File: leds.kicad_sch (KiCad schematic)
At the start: 12 parts

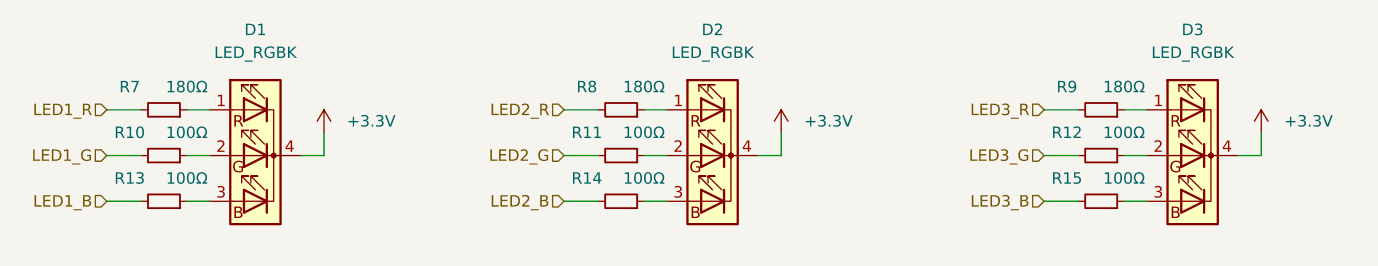
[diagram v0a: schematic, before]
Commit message: Improve DCDC converter diagram
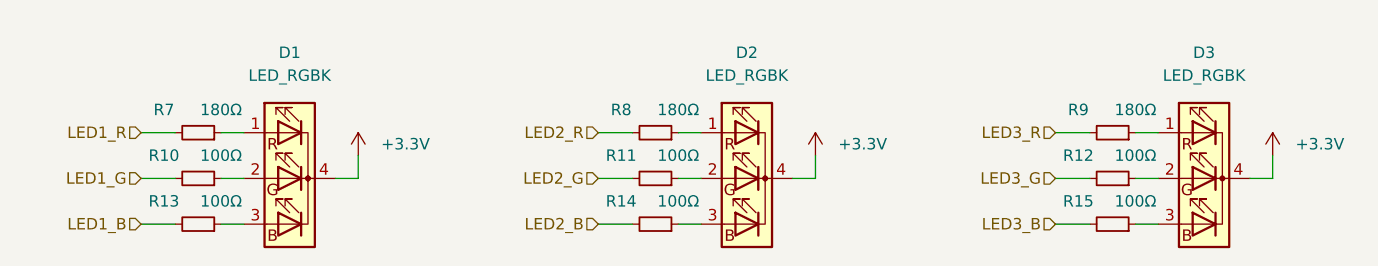
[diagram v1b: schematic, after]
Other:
- company: (none) -> Authors: A. Kotkov, I. Kajdan
- title: (none) -> Debug LEDs
- moved on the sheet: D1, D2, D3, R10, R11, R12, R13, R14, R15, R7, R8, R9
